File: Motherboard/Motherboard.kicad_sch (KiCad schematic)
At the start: 69 parts, among them J1 ATX-20, J2 65SIB_Connector, J3 DB9_Header, J4 GPIO_Connector, J5 Expansion_Connector, J6 Expansion_Connector, J7 Expansion_Connector, J8 Expansion_Connector, J9 Expansion_Connector, SW1 SW_SPST, U1 74HCT138, U2 AS6C4008-55PCN, U3 ATF22V10C, U4 DS1813, U6 28C010, X1 ACO-8MHz

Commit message: 150 unrouted traces...
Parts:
- removed C20, C21, C22, C23, C24, C25, C26, C27: 100 nF, Capacitor_THT:C_Disc_D3.0mm_W1.6mm_P2.50mm, symbol Device:C
- removed U1: 74HCT138, Package_DIP:DIP-16_W7.62mm_Socket_LongPads, symbol 74xx:74LS138
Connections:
- net ~{CS_UART} is gone; now on net ~{CS_GPIO}: U3.15 (I/O), UART-RS232.20 (~{En}), UART1.3 (~{CS1})
- net CS_DEV: no longer 65SIB_LATCH1.6 (E2), GPIO_CTRL1.24 (CS1), J5.28 (Pin_28), J6.28 (Pin_28), J7.28 (Pin_28), J8.28 (Pin_28), J9.28 (Pin_28), U3.14 (I/O), UART1.2 (CS0)
- net VCC: now also 65SIB_LATCH1.6 (E2), GPIO_CTRL1.24 (CS1), UART1.2 (CS0)
- net ~{CS_65SIB}: now also U3.16 (I/O); no longer U3.17 (I/O)
- net ~{CS_GPIO}: now also U3.14 (I/O); no longer U3.16 (I/O)

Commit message: 104 unrouted traces...
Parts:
- 65SIB/MM1, GPIO_CTRL1: value WD65C22 -> WD65C22N
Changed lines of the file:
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@@
       (effects (font (size 1.524 1.524)))
     )
-    (property "Value" "WD65C22" (id 1) (at 76.2 245.5926 0)
+    (property "Value" "WD65C22N" (id 1) (at 76.2 245.5926 0)
       (effects (font (size 1.524 1.524)))
     )
@@
       (effects (font (size 1.524 1.524)))
     )
-    (property "Value" "WD65C22" (id 1) (at 411.48 52.5526 0)
+    (property "Value" "WD65C22N" (id 1) (at 411.48 52.5526 0)
       (effects (font (size 1.524 1.524)))
     )
@@
     )
     (path "/00000000-0000-0000-0000-000061c6031f"
-      (reference "65SIB/MM1") (unit 1) (value "WD65C22") (footprint "Package_DIP:DIP-40_W15.24mm_Socket_LongPads")
+      (reference "65SIB/MM1") (unit 1) (value "WD65C22N") (footprint "Package_DIP:DIP-40_W15.24mm_Socket_LongPads")
     )
     (path "/00000000-0000-0000-0000-00006343fd00"
@@
     )
     (path "/00000000-0000-0000-0000-000061a772a1"
-      (reference "GPIO_CTRL1") (unit 1) (value "WD65C22") (footprint "Package_DIP:DIP-40_W15.24mm_Socket_LongPads")
+      (reference "GPIO_CTRL1") (unit 1) (value "WD65C22N") (footprint "Package_DIP:DIP-40_W15.24mm_Socket_LongPads")
     )
     (path "/00000000-0000-0000-0000-00006483e48f"

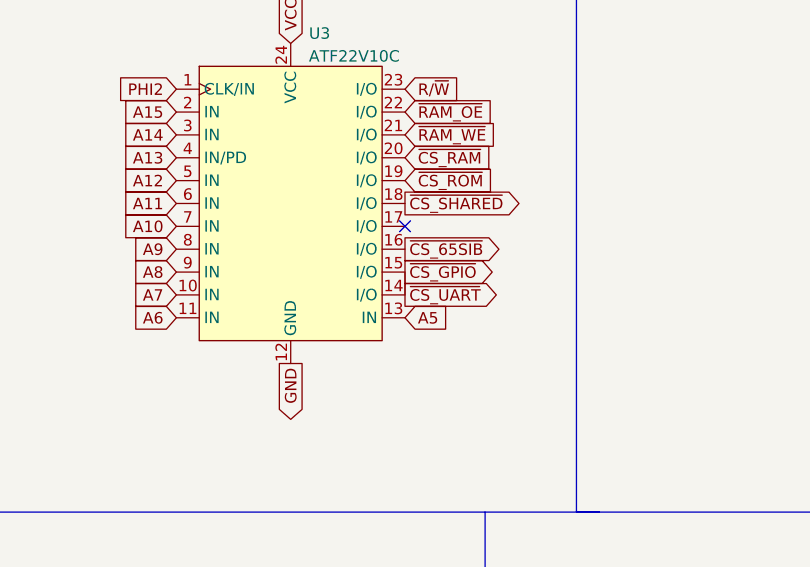
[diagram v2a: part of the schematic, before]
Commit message: Completed version 2.6...
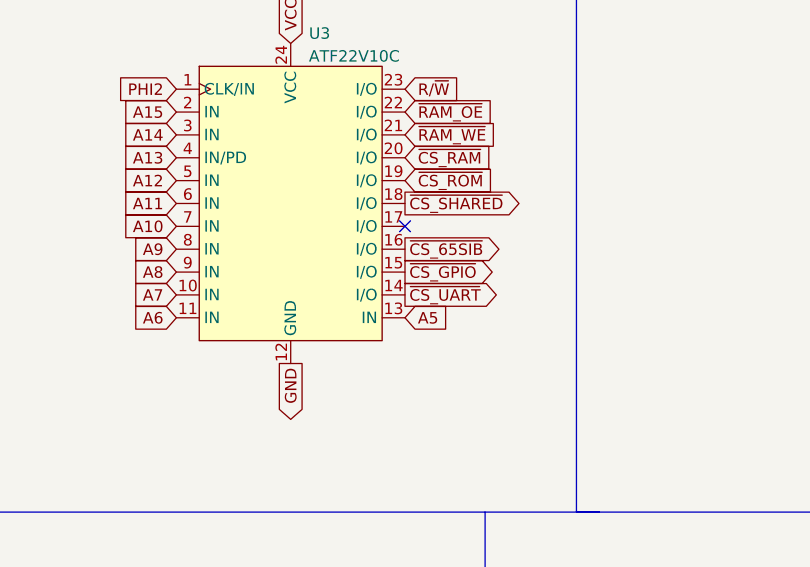
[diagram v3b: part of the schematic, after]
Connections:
- net ~{CS_GPIO}: no longer U3.14 (I/O), UART-RS232.20 (~{En}), UART1.3 (~{CS1})
- new net ~{CS_UART}: U3.14 (I/O), UART-RS232.20 (~{En}), UART1.3 (~{CS1})
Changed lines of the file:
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@@
-    (stroke (width 0) (type default) (color 0 0 0 0))
-  )
-  (wire (pts (xy 474.98 157.48) (xy 474.98 154.94))
     (stroke (width 0) (type default) (color 0 0 0 0))
   )
